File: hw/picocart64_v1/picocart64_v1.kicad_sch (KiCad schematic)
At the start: 0 parts

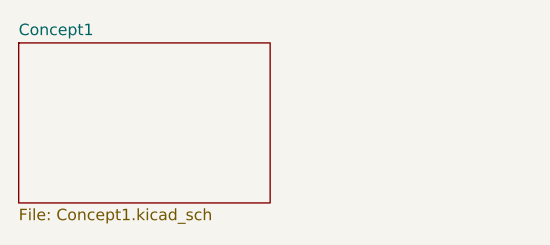
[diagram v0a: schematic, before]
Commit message: hw: Concept2, is this the future?
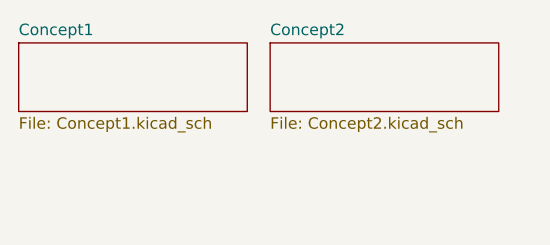
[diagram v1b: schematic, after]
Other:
- added sheet Concept2 (Concept2.kicad_sch)
